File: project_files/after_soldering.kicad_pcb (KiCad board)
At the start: 2 copper layers, 95.3 x 104.8 mm, 48 parts, among them SW11 SW_Push, SW12 SW_Push, SW13 SW_Push, SW17 SW_Push, SW18 SW_Push, SW19 SW_Push, SW3 SW_Push, SW4 SW_Push, SW5 SW_Push, SW7 SW_Push, SW8 SW_Push, SW9 SW_Push, U1 MOUDLE-SEEEDUINO-XIAO

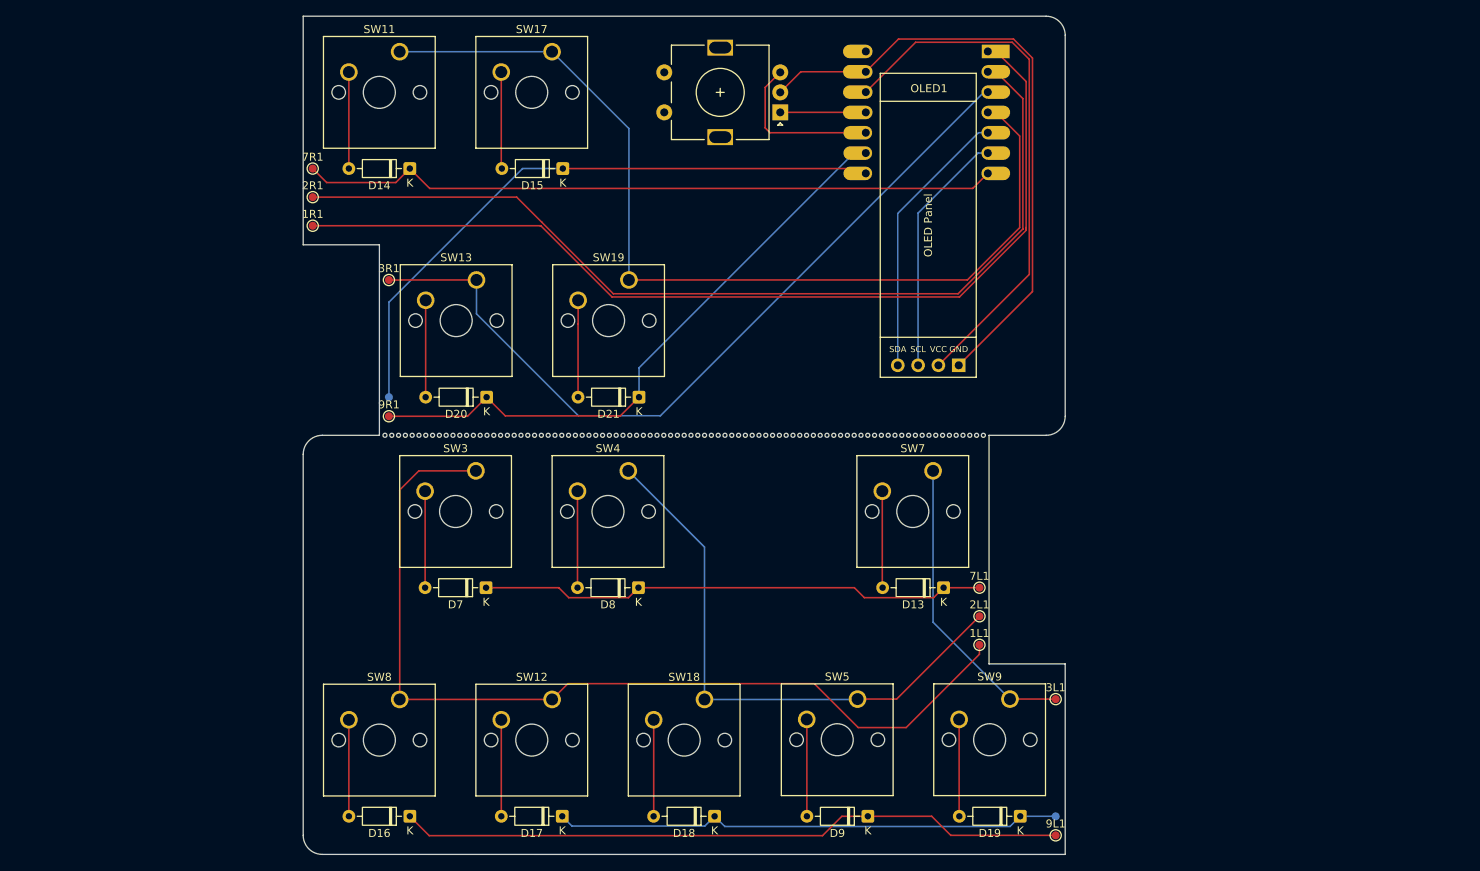
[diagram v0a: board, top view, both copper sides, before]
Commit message: after solder
and curves :)
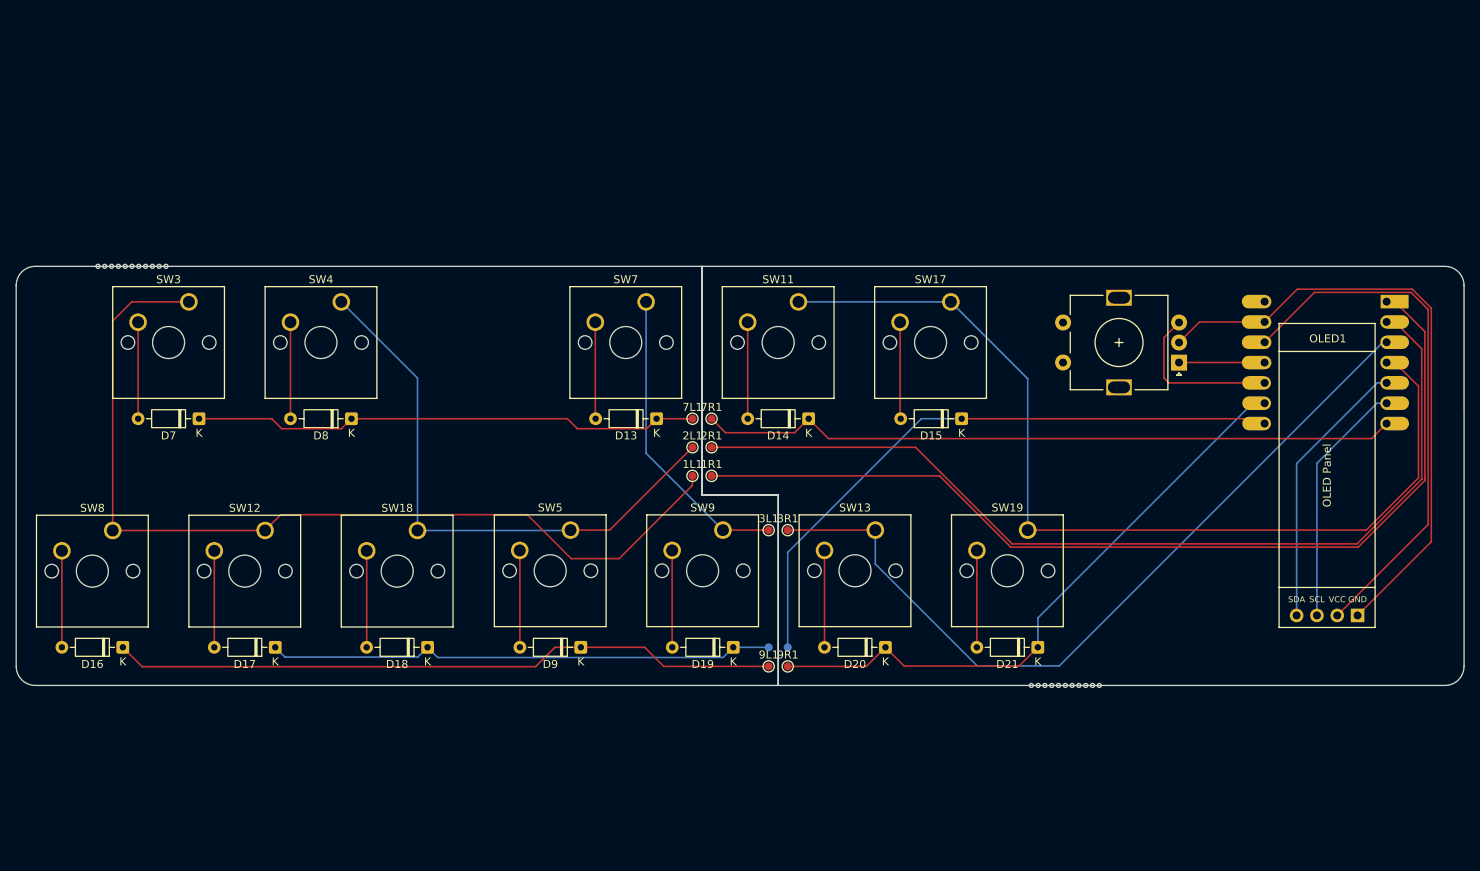
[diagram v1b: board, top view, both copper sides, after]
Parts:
- removed the REF** at (175.2, 90.5)
- removed the REF** at (128.4, 90.5)
- removed the REF** at (137.8, 90.5)
- removed the REF** at (119.1, 90.5)
- removed the REF** at (180.3, 90.5)
- removed the REF** at (165.8, 90.5)
- removed the REF** at (156.5, 90.5)
- removed the REF** at (147.1, 90.5)
- added REF**: BreakLine_11h_D0.5mm_P0.85mm, Panelization:BreakLine_11h_D0.5mm_P0.85mm, F.Cu at (190.5, 121.8)
- moved 3R1 58.8 mm to (155.8, 102.3)
- moved 7R1 58.8 mm to (146.3, 88.4)
- moved D14 58.8 mm to (158.4, 88.4)
- moved D15 58.8 mm to (177.6, 88.4)
- moved D21 58.8 mm to (187.1, 117.0)
- moved SW17 58.8 mm to (176.2, 73.8)
- moved SW19 58.8 mm to (185.8, 102.3)
- moved 1R1 58.8 mm to (146.3, 95.6)
- moved 2R1 58.8 mm to (146.3, 92.0)
- moved 8R1 58.8 mm to (155.8, 117.0)
- moved 9R1 58.8 mm to (155.8, 119.4)
- moved D20 58.8 mm to (168.0, 117.0)
- moved OLED1 58.8 mm to (229.2, 76.5)
- moved SW11 58.8 mm to (157.2, 73.8)
- moved SW13 58.8 mm to (166.8, 102.3)
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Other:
- board size 95.3 x 104.8 mm -> 181 x 52.4 mm

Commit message: oled centered
with silkscreen!
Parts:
- moved 1R1 173.6 mm to (-8.33, 16.7)
- moved 2L1 173.6 mm to (-10.7, 13.1)
- moved 2R1 173.6 mm to (-8.33, 13.1)
- moved 3L1 173.6 mm to (-1.19, 23.5)
- moved 3R1 173.6 mm to (1.20, 23.5)
- moved 7L1 173.6 mm to (-10.7, 9.53)
- moved 7R1 173.6 mm to (-8.33, 9.53)
- moved 8L1 173.6 mm to (-1.19, 38.1)
- moved 8R1 173.6 mm to (1.20, 38.1)
- moved 9L1 173.6 mm to (-1.19, 40.5)
- moved 9R1 173.6 mm to (1.20, 40.5)
- moved D13 173.6 mm to (-15.2, 9.53)
- moved D14 173.6 mm to (3.81, 9.53)
- moved D15 173.6 mm to (22.9, 9.53)
- moved D16 173.6 mm to (-81.9, 38.1)
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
